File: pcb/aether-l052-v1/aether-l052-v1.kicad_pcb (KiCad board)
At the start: 2 copper layers, 50.8 x 22.9 mm, 40 parts, among them J1 USB_C_Receptacle_USB2.0_16P, J2 Conn_01x16_Pin, J3 Conn_01x12_Pin, J4 S2B-PH-SM4-TB, J5 BM04B-SRSS-TB, J6 Conn_ARM_JTAG_SWD_10, Q1 DMG2305UX-7, U1 MCP1711T-3.3I/OT, U2 MCP73832-2-OT, U3 STM32L052K8Ux

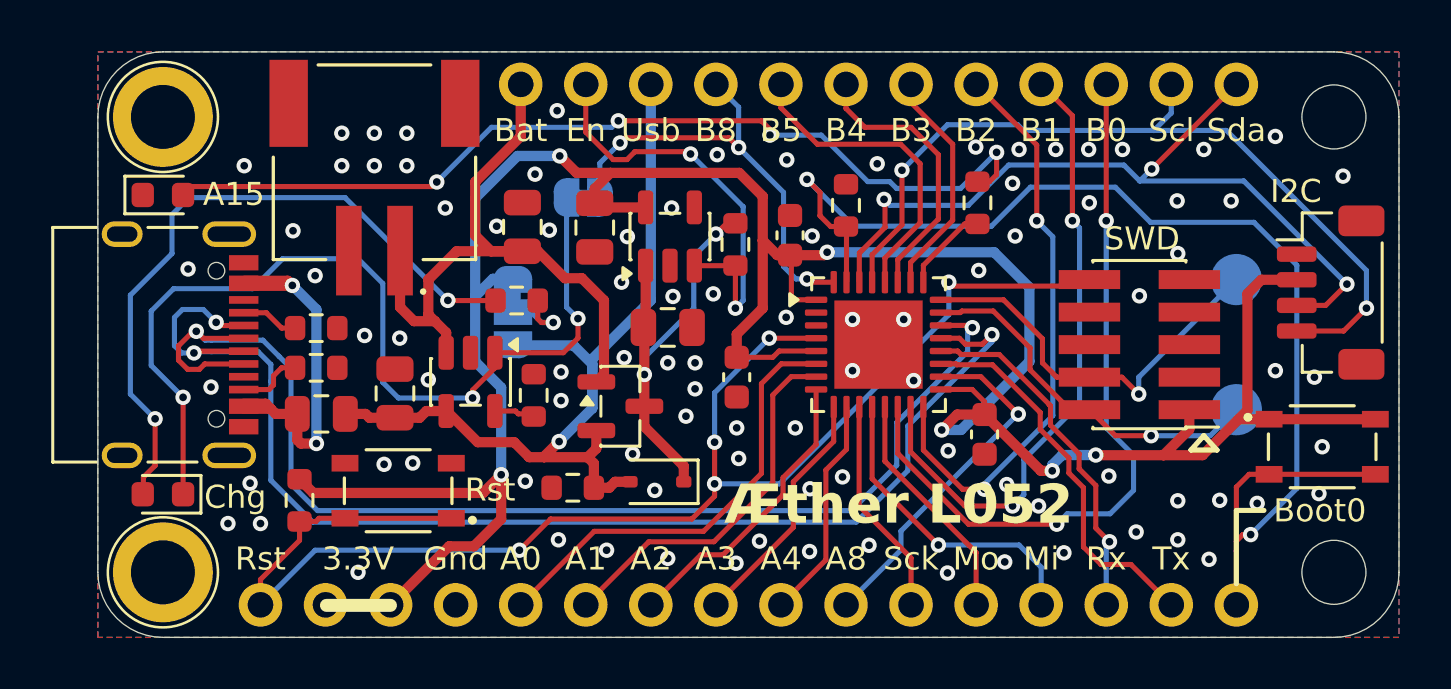
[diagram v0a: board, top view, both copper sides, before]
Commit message: finishing board, add gerber, bom, cpl
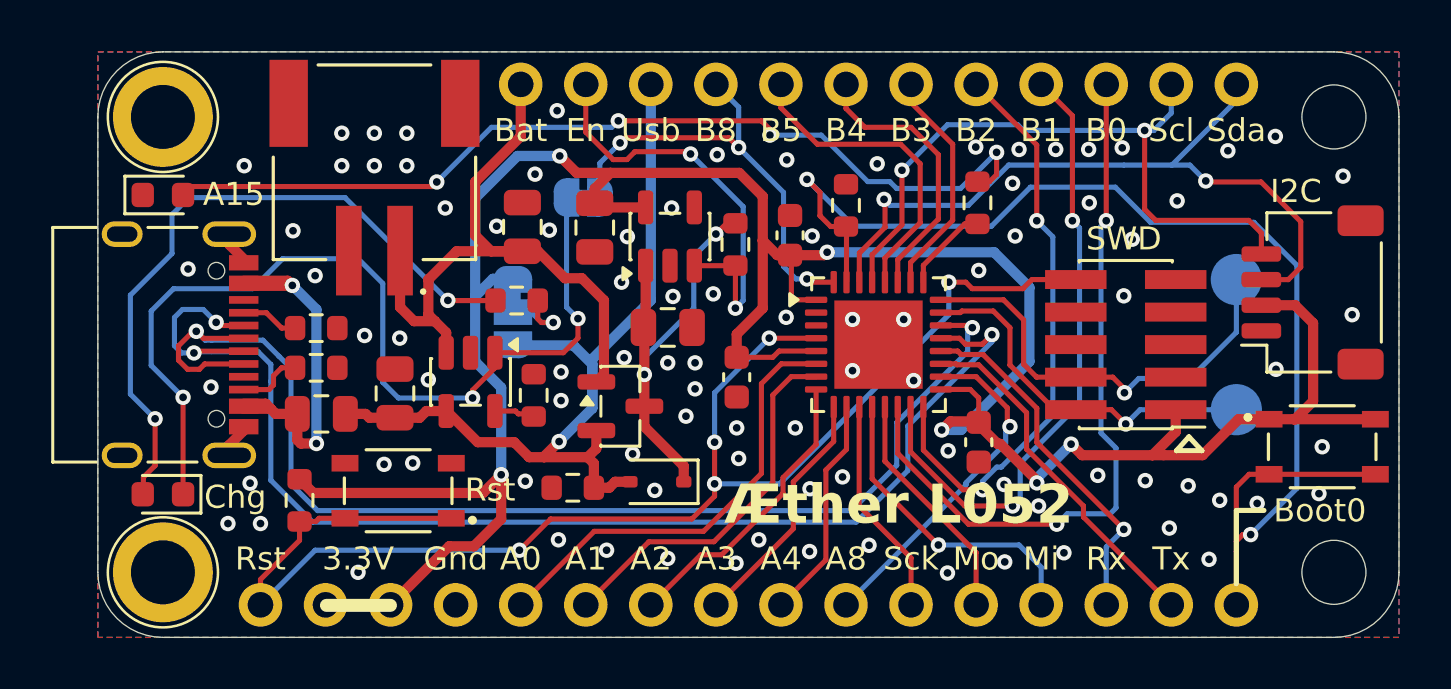
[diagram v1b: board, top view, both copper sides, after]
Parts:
- J5: value BM04B-SRSS-TB -> SM04B-SRSS-TB; footprint Connector_JST:JST_SH_BM04B-SRSS-TB_1x04-1MP_P1.00mm_Vertical -> Connector_JST:JST_SH_SM04B-SRSS-TB_1x04-1MP_P1.00mm_Horizontal
- moved J5 0.71 mm to (149.0, 88.1), turned to 90 degrees
- moved J6 0.53 mm to (141.7, 90.2)
- moved C5 0.38 mm to (136.0, 94.0)
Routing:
- net /B6_I2C1_SCL: track 32.9 -> 26.6 mm
- net GND: track 0.00 -> 2.96 mm, vias 94 -> 93
- net /B7_I2C1_SDA: track 32.2 -> 29.3 mm, vias 3 -> 2
- net /SWCLK: track 15.8 -> 17.2 mm
- net /A9_USART1_TX: track 15.0 -> 14.0 mm
